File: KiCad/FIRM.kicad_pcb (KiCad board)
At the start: 4 copper layers, 40.5 x 40.5 mm, 98 parts, among them J2 DM3CS-SF, Q2 IRLML6402, U1 STM32F405RGTx, U2 MIC5219-3.3YM5, U6 A-USBC-20F0-EA-GSR05, U7 W25Q128JVS, X2 32.768khz, Y1 12 MHz

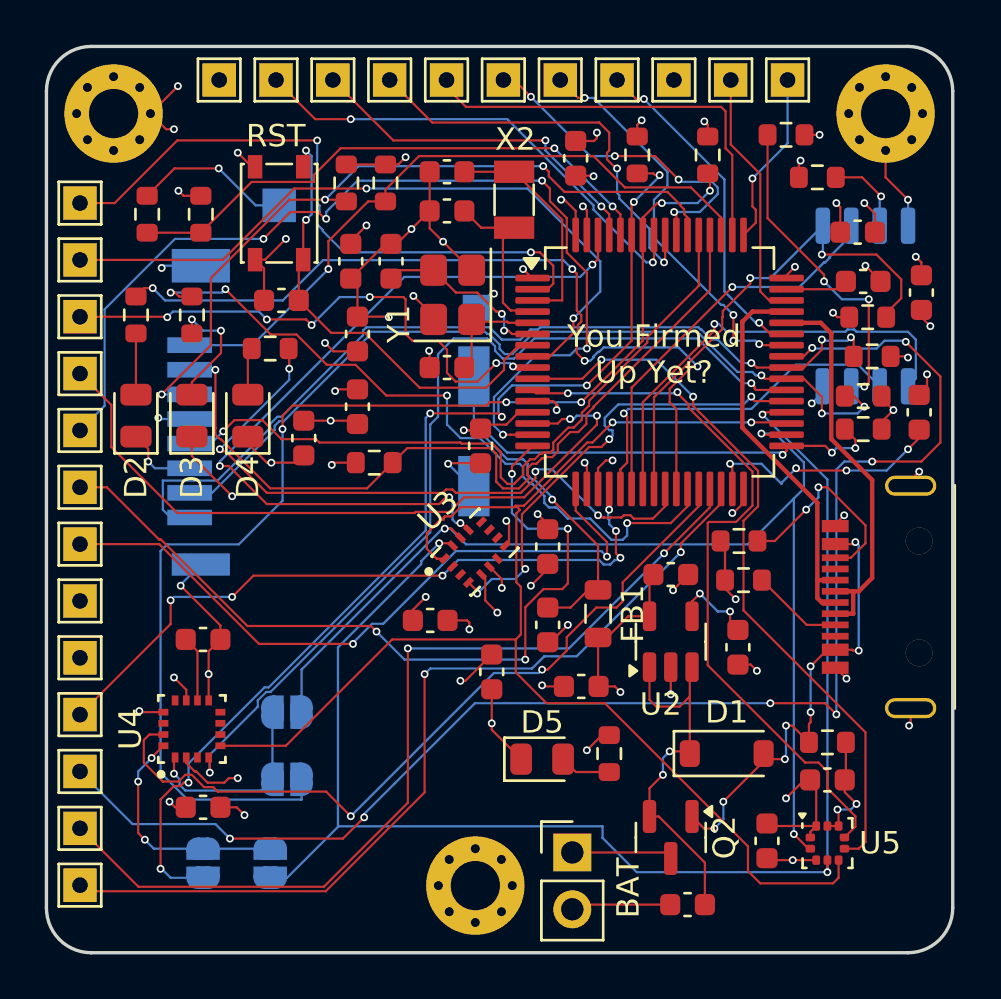
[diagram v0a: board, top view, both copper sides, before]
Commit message: refine traces
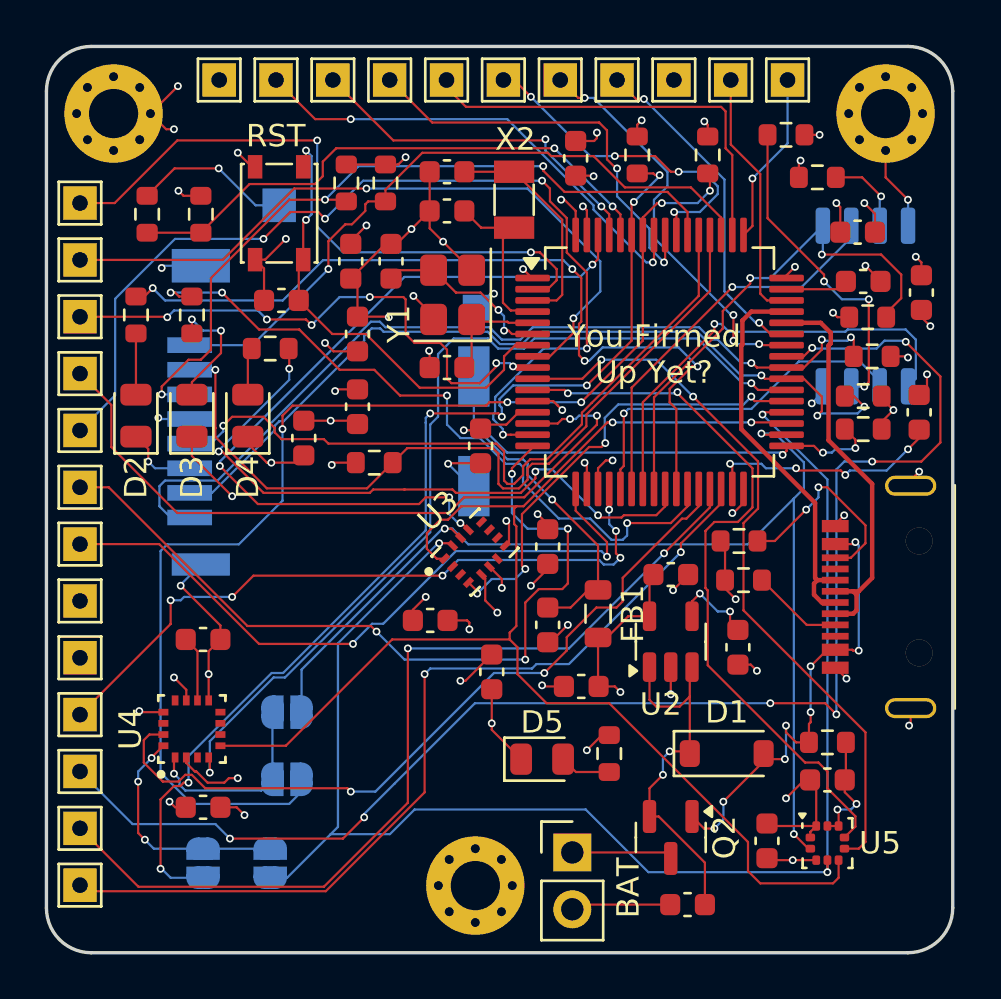
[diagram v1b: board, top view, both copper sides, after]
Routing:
- net /MOSI2: track 65.5 -> 66.3 mm
- net /MAG_INT: track 35.4 -> 34.6 mm
